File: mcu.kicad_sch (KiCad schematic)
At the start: 12 parts, among them U1 STM32F405RGTx, Y1 8M

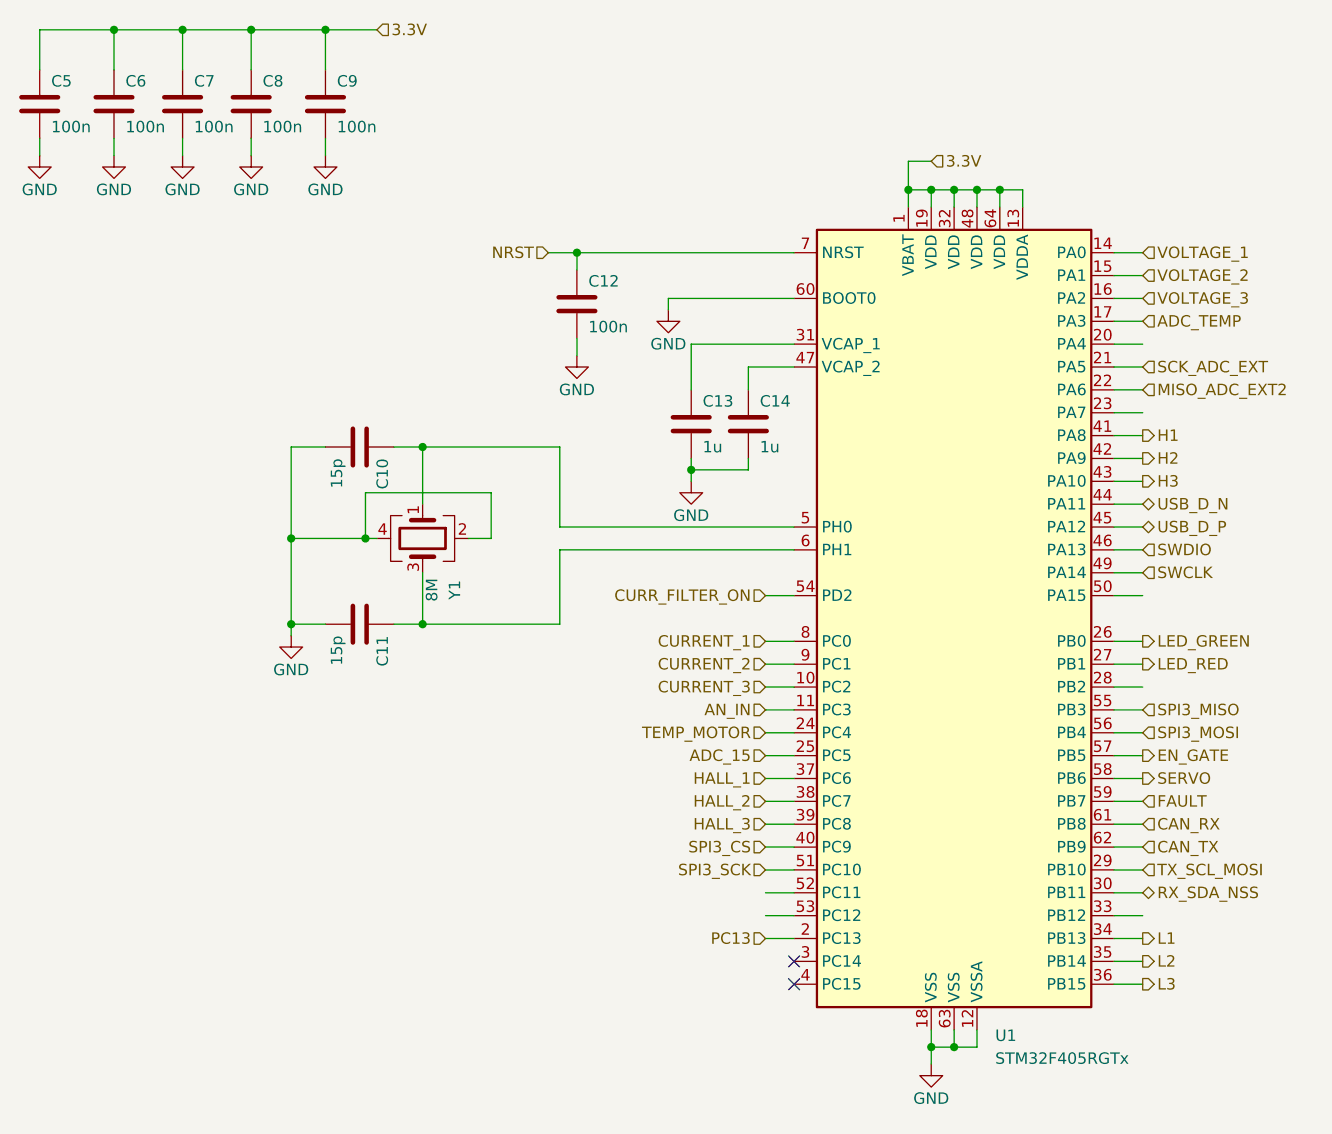
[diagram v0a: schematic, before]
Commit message: Update
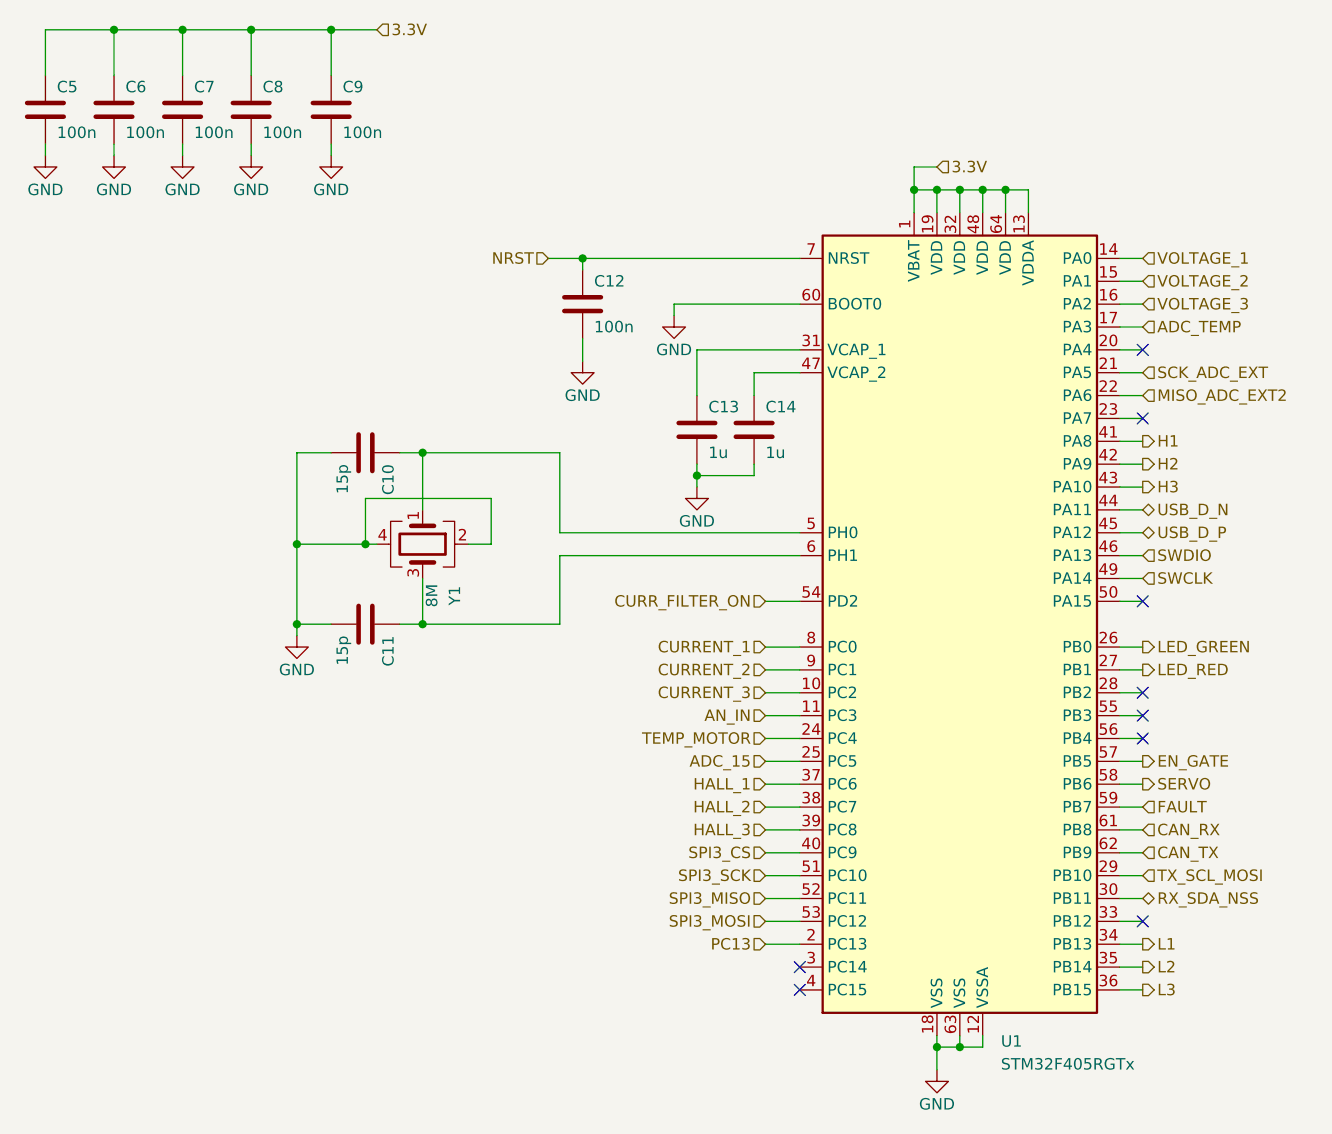
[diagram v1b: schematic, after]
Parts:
- C12, C5, C6, C7, C8, C9: Voltage 50V -> 100V
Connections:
- net SPI3_MISO: now also U1.52 (PC11); no longer U1.55 (PB3)
- net SPI3_MOSI: now also U1.53 (PC12); no longer U1.56 (PB4)
- no-connect marks 2 -> 9
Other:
- moved on the sheet: C10, C11, C12, C13, C14, C5, C6, C7, C8, C9, U1, Y1
